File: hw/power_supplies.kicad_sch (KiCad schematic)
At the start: 21 parts, among them IC4 AZ1117CR-3.3TRG1, U10 LNK306DN-TL

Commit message: update comments
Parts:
- C10, C9: Manufacturer_Name (none) -> Murata; Manufacturer_Part_Number (none) -> GRT188C81E475KE13D
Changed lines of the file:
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@@
+      (effects (font (size 1.27 1.27)) hide)
+    )
+    (property "Manufacturer_Name" "Murata" (id 4) (at 38.1 161.29 0)
+      (effects (font (size 1.27 1.27)) hide)
+    )
+    (property "Manufacturer_Part_Number" "GRT188C81E475KE13D " (id 5) (at 38.1 161.29 0)
       (effects (font (size 1.27 1.27)) hide)
     )
@@
       (effects (font (size 1.27 1.27)) hide)
     )
+    (property "Manufacturer_Name" "Murata" (id 4) (at 38.1 113.03 0)
+      (effects (font (size 1.27 1.27)) hide)
+    )
+    (property "Manufacturer_Part_Number" "GRT188C81E475KE13D " (id 5) (at 38.1 113.03 0)
+      (effects (font (size 1.27 1.27)) hide)
+    )

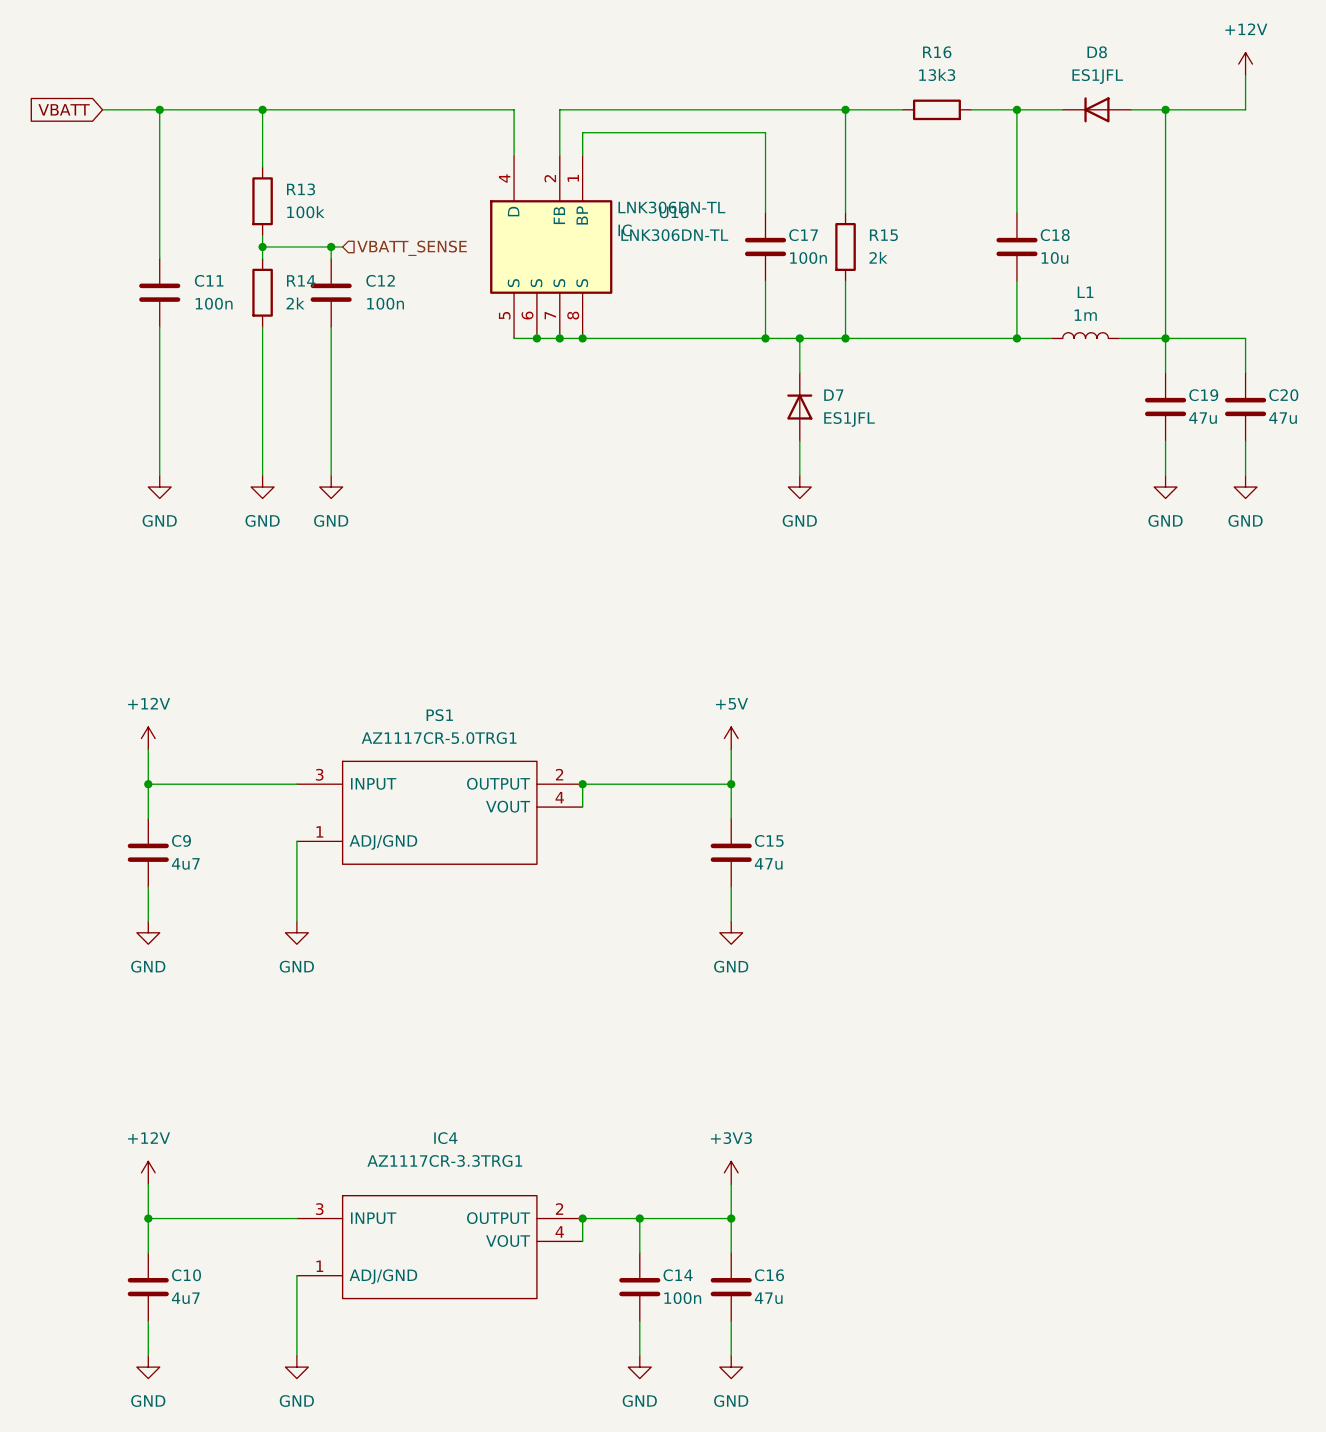
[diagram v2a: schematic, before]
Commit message: commenting
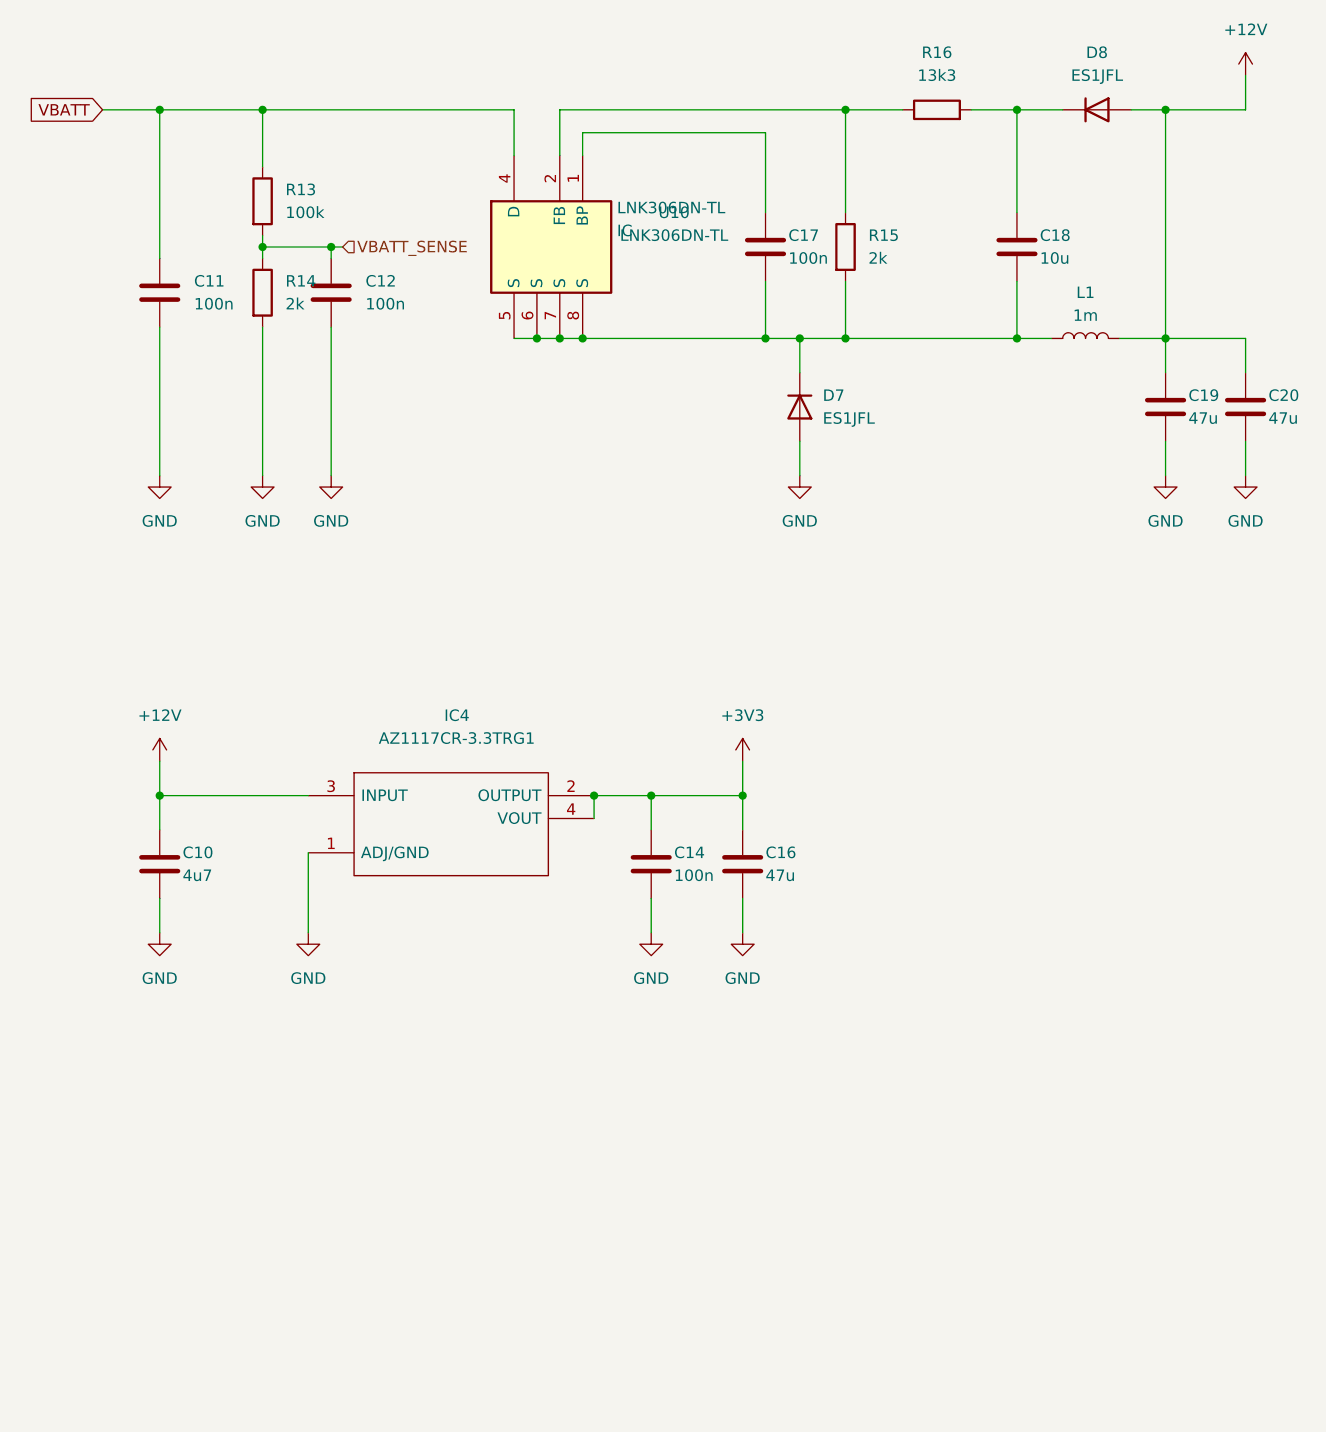
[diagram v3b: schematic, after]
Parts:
- removed C15: 47u, Capacitor_SMD:C_1210_3225Metric, symbol Device:C
- removed C9: 4u7, Capacitor_SMD:C_0603_1608Metric, symbol Device:C
- removed PS1: AZ1117CR-5.0TRG1, MAG_LDO_Regulators:AZ1117CR33TRG1, symbol MAG_LDO_Regulators:AZ1117CR-5.0TRG1
- U10: footprint MAG_Switching_Regulators:SOIC127P600X175-8N -> MAG_Switching_Regulators:SOIC127P600X175-8N_MISSING_PIN
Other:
- moved on the sheet: C10, C14, C16, IC4
